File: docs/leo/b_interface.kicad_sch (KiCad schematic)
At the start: 8 parts, among them IC37 74LS245, IC38 74LS244, IC39 74LS374, IC40 74LS245, IC46 74LS161, IC47 GAL16V8, IC48 74LS374, IC49 74LS244

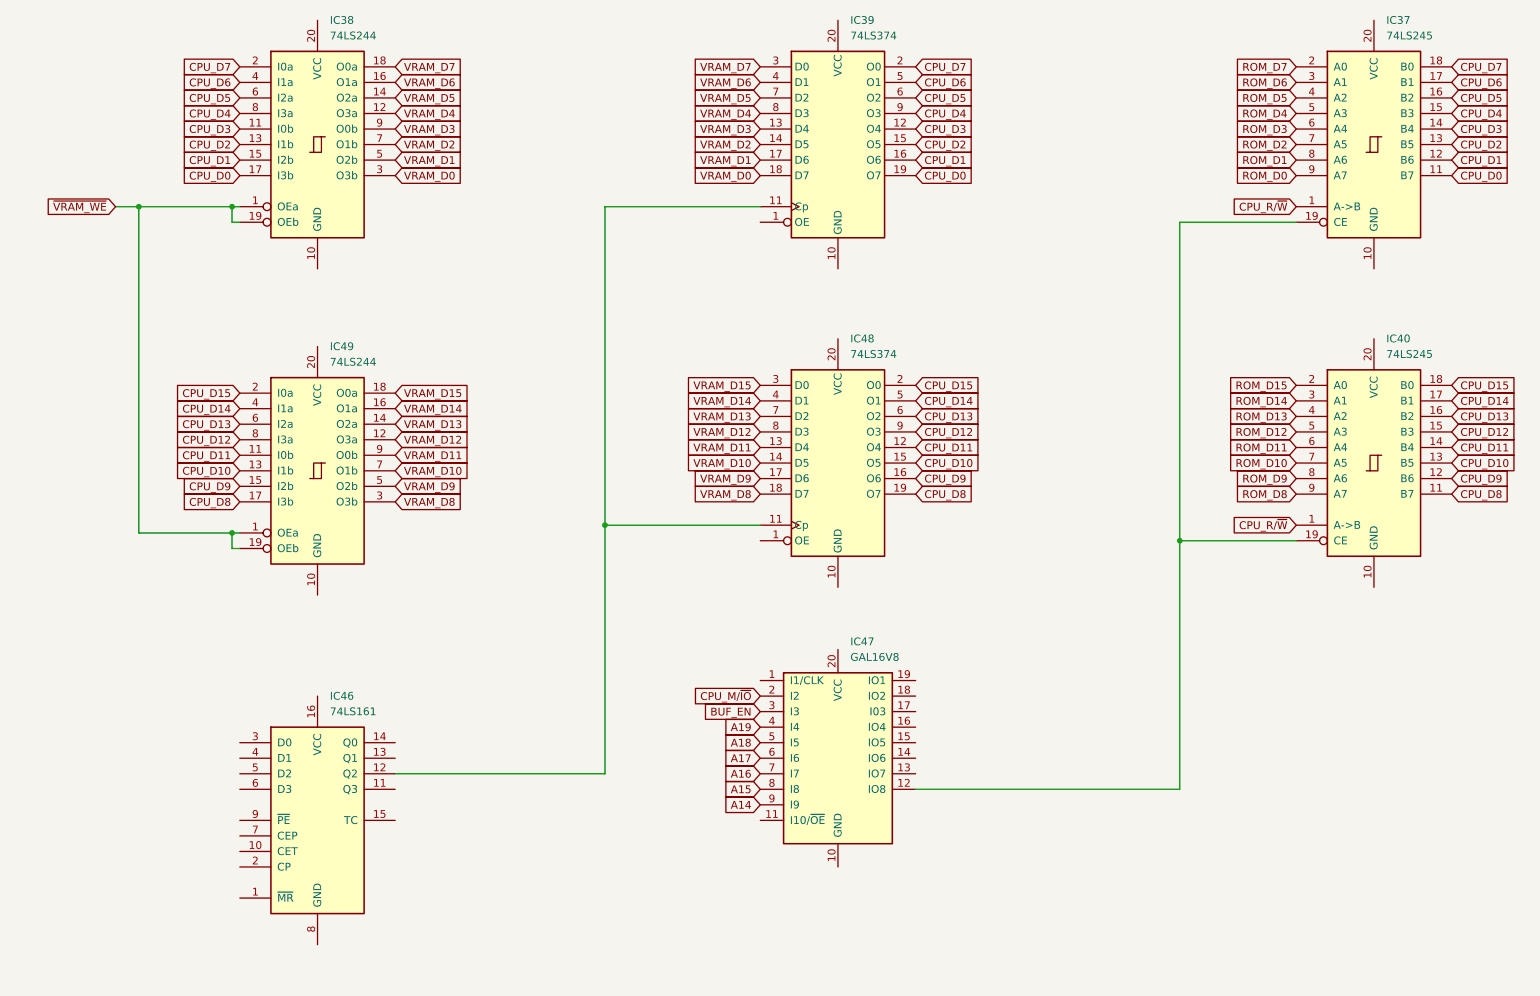
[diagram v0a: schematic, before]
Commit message: Add more b board logic
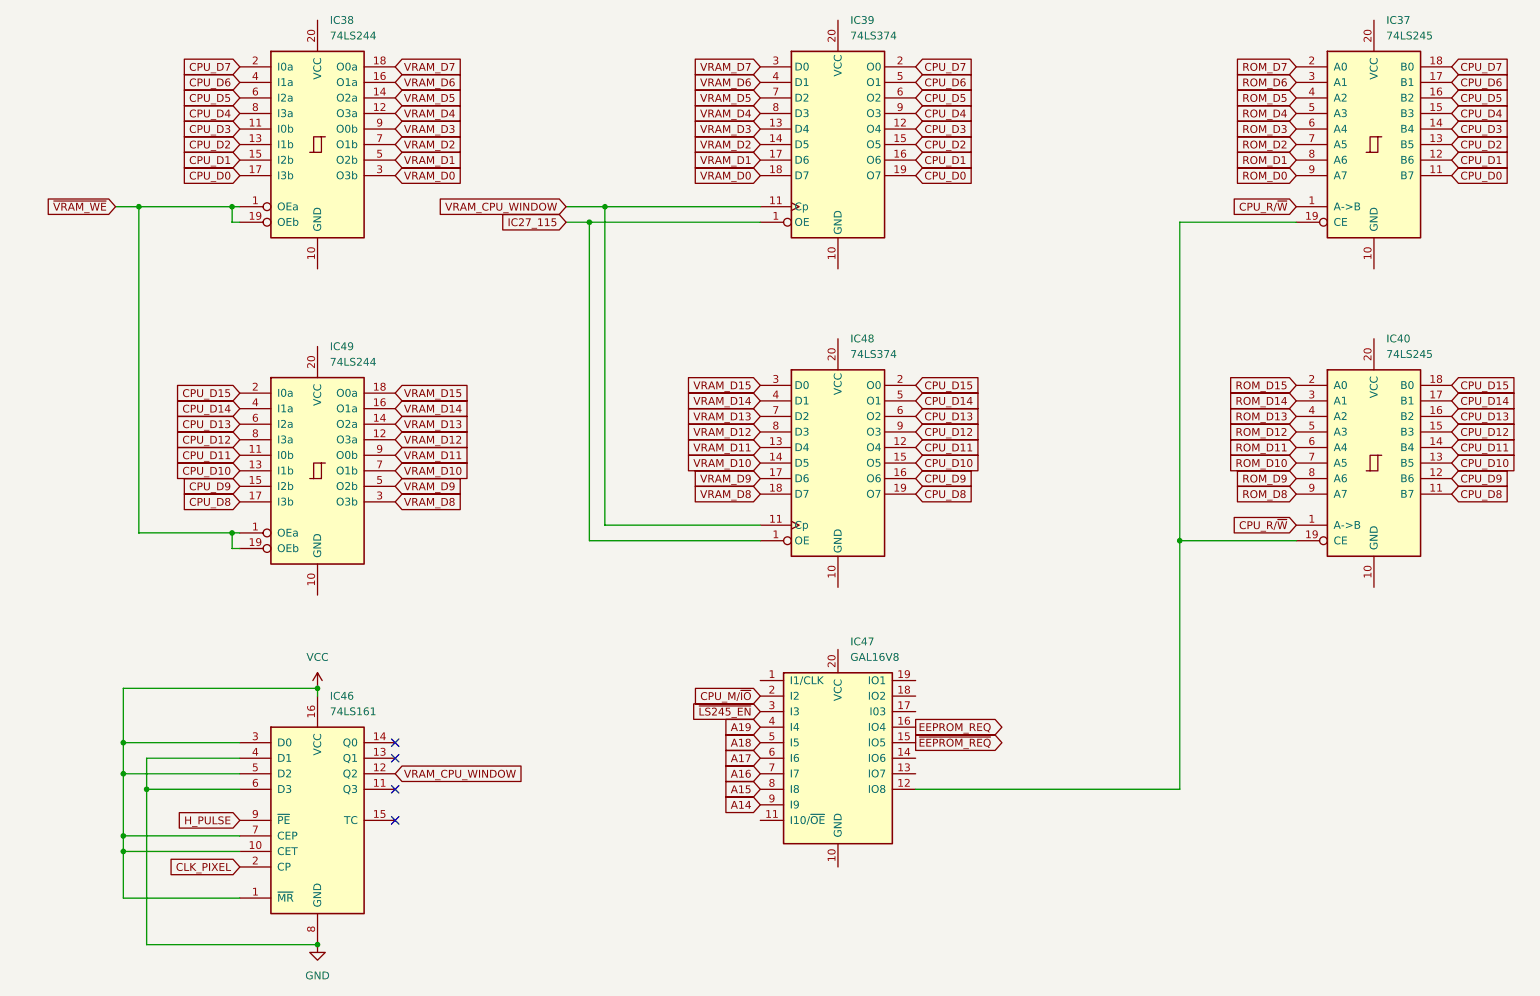
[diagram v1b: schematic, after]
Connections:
- net ~{EEPROM_REQ}: now reaches IC47.15 (IO5)
- net EEPROM_REQ: now reaches IC47.16 (IO4)
- net IC27_115: now reaches IC48.1 (OE)
- net IC27_115: now also IC39.1 (OE)
- net VRAM_CPU_WINDOW: now reaches IC39.11 (Cp), IC46.12 (Q2), IC48.11 (Cp)
- net VCC: now reaches IC46.1 (~{MR})
- net VCC: now also IC46.10 (CET), IC46.16 (VCC), IC46.3 (D0), IC46.5 (D2), IC46.7 (CEP)
- net CLK_PIXEL: now reaches IC46.2 (CP)
- net GND: now reaches IC46.4 (D1)
- net GND: now also IC46.6 (D3), IC46.8 (GND)
- net H_PULSE: now reaches IC46.9 (~{PE})
- net BUF_EN renamed ~{LS245_EN}
- no-connect marks 0 -> 4
